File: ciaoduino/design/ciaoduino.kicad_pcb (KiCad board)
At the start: 2 copper layers, 58.4 x 37.3 mm, 17 parts, among them P1 ICSP, P2 CONN_01X02, P3 USB_OTG, P4 CONN_01X06, P5 CONN_01X06, P6 CONN_01X04, P7 CONN_01X14, SW1 SW_PUSH, SW2 SW_PUSH, U2 ATmega32U4-AU, X1 CRYSTAL_SMD

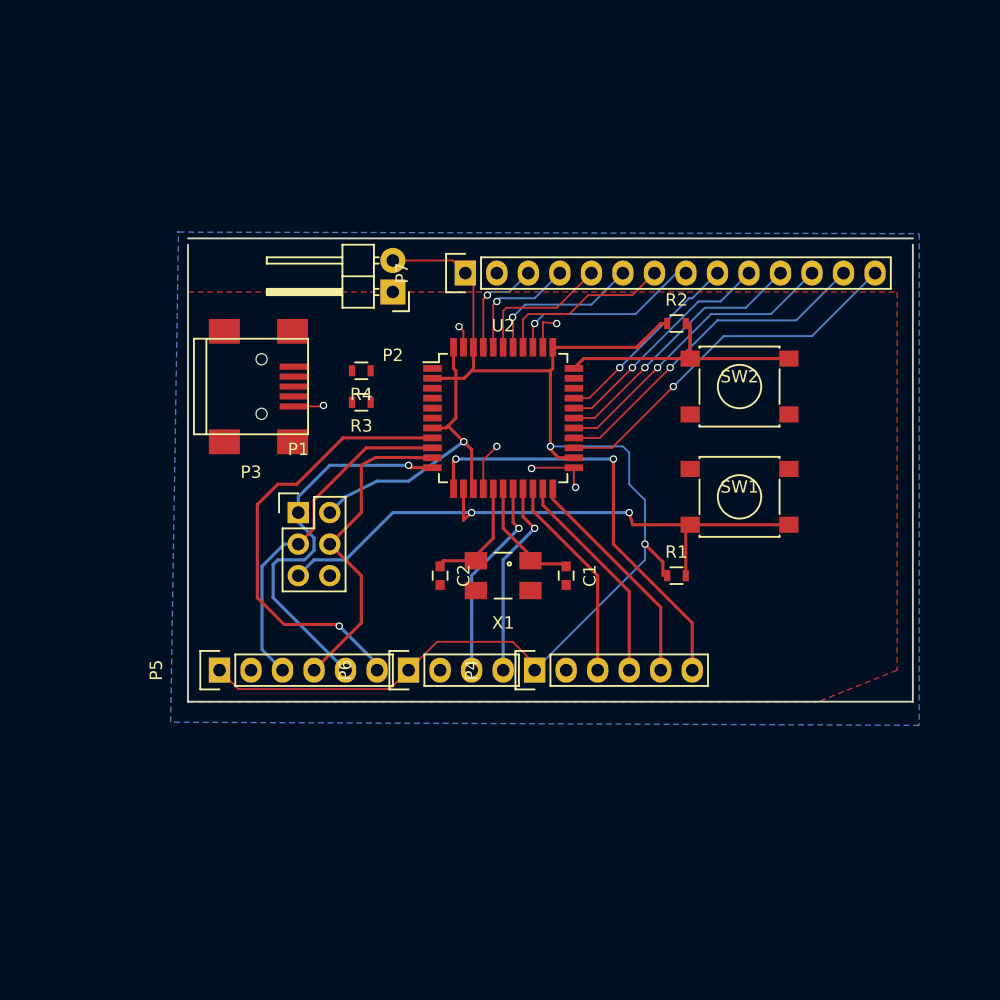
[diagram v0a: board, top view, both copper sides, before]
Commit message: Rework layout.
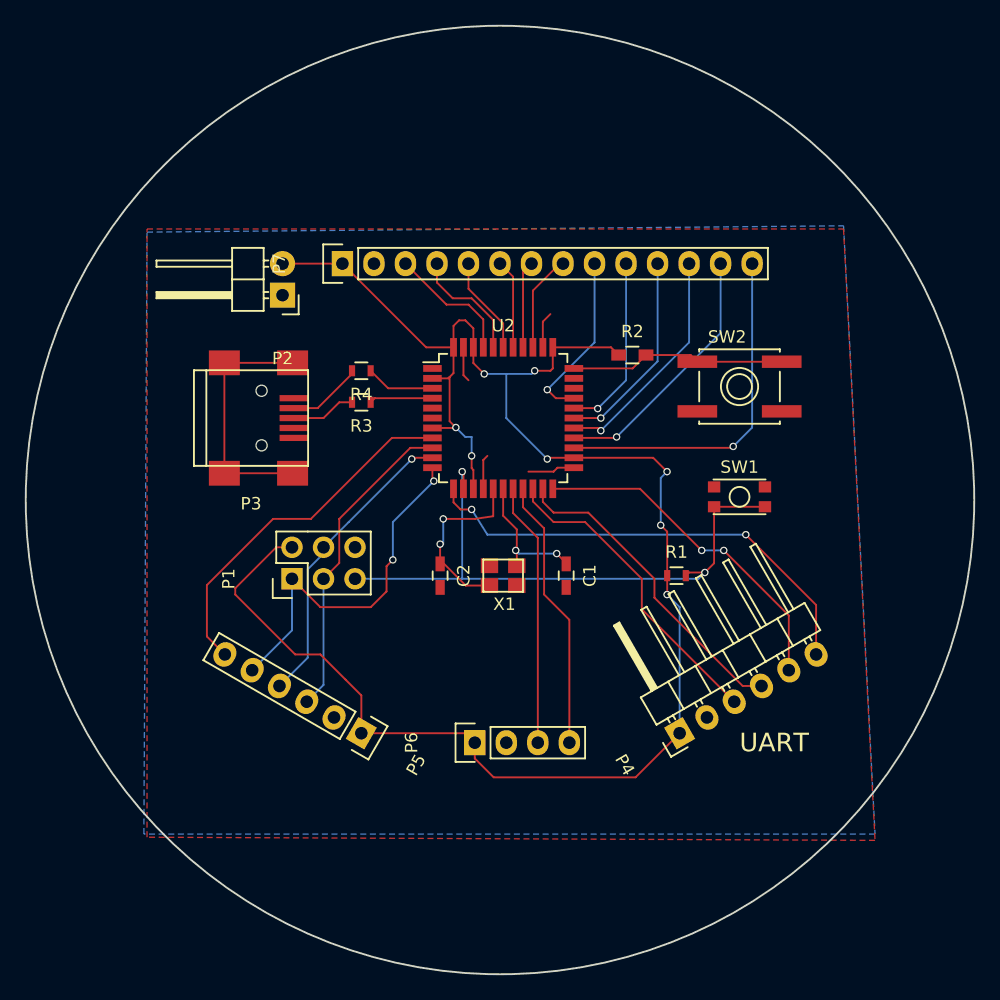
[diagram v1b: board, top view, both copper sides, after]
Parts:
- C1, C2: footprint Capacitors_SMD:C_0603 -> Capacitors_SMD:C_0603_HandSoldering
- P4: footprint Pin_Headers:Pin_Header_Straight_1x06 -> Pin_Headers:Pin_Header_Angled_1x06
- R2: footprint Resistors_SMD:R_0603 -> Resistors_SMD:R_0603_HandSoldering
- SW1: footprint Buttons_Switches_SMD:SW_SPST_PTS645 -> Buttons_Switches_SMD:SW_SPST_KMR2
- SW2: footprint Buttons_Switches_SMD:SW_SPST_PTS645 -> Buttons_Switches_SMD:SW_SPST_EVQP0
- X1: footprint Crystals:Crystal_SMD_0603_4Pads -> Crystals:crystal_FA238-TSX3225
- moved P4 12.7 mm to (165.4, 100.3), turned to 120 degrees
- moved P5 12.5 mm to (139.7, 100.3), turned to 240 degrees
- moved P7 9.94 mm to (138.2, 62.5)
- moved P2 8.89 mm to (133.3, 65.0)
- moved P6 7.91 mm to (148.8, 101.1)
- moved P1 5.36 mm to (134.1, 87.9), turned to 90 degrees
- moved R2 4.37 mm to (161.5, 69.8)
- moved P3 2.54 mm to (130.8, 74.9)
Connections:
- P3 pad 1: Net-(P3-Pad1) -> (no net)
- P3 pad 4: Net-(P3-Pad4) -> (no net)
- U2 pad 1: Net-(U2-Pad1) -> (no net)
- U2 pad 31: Net-(U2-Pad31) -> (no net)
- U2 pad 32: Net-(U2-Pad32) -> (no net)
- U2 pad 5: Net-(U2-Pad5) -> (no net)
- U2 pad 6: Net-(U2-Pad6) -> (no net)
- X1 pad 3: Net-(X1-Pad3) -> GND
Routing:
- net Net-(P3-Pad6): track 0.00 -> 19.9 mm
- net VCC: track 132.5 -> 146.0 mm, vias 3 -> 8
- net usart_cts: track 18.2 -> 27.7 mm, vias 0 -> 2
- net usart_rx: track 16.8 -> 25.4 mm
- net usart_tx: track 17.5 -> 25.7 mm
- net ADC7: track 15.9 -> 7.90 mm, vias 1 -> 0
- net ADC6: track 14.4 -> 7.03 mm
- net SS: track 36.2 -> 29.3 mm, vias 1 -> 0
- net ADC9: track 27.2 -> 20.9 mm
- net Net-(P3-Pad2): track 0.00 -> 6.08 mm
- net Net-(R2-Pad2): track 23.5 -> 17.4 mm
- net SDA: track 16.1 -> 22.0 mm, vias 1 -> 0
- net ADC10: track 24.4 -> 18.7 mm
- net ADC5: track 12.8 -> 7.18 mm, vias 1 -> 0
- net Net-(R4-Pad1): track 0.00 -> 5.56 mm
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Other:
- board size 58.4 x 37.3 mm -> 76.4 x 76.4 mm
- board text added: "UART"
